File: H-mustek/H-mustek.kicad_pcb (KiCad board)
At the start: 2 copper layers, 22 parts, among them J1 Conn_01x02_Pin, J2 Conn_01x02_Pin, Q1 IRF3205, Q2 IRF3205, Q3 IRF3205, Q4 IRF3205, U1 IR2153, U2 IR2153

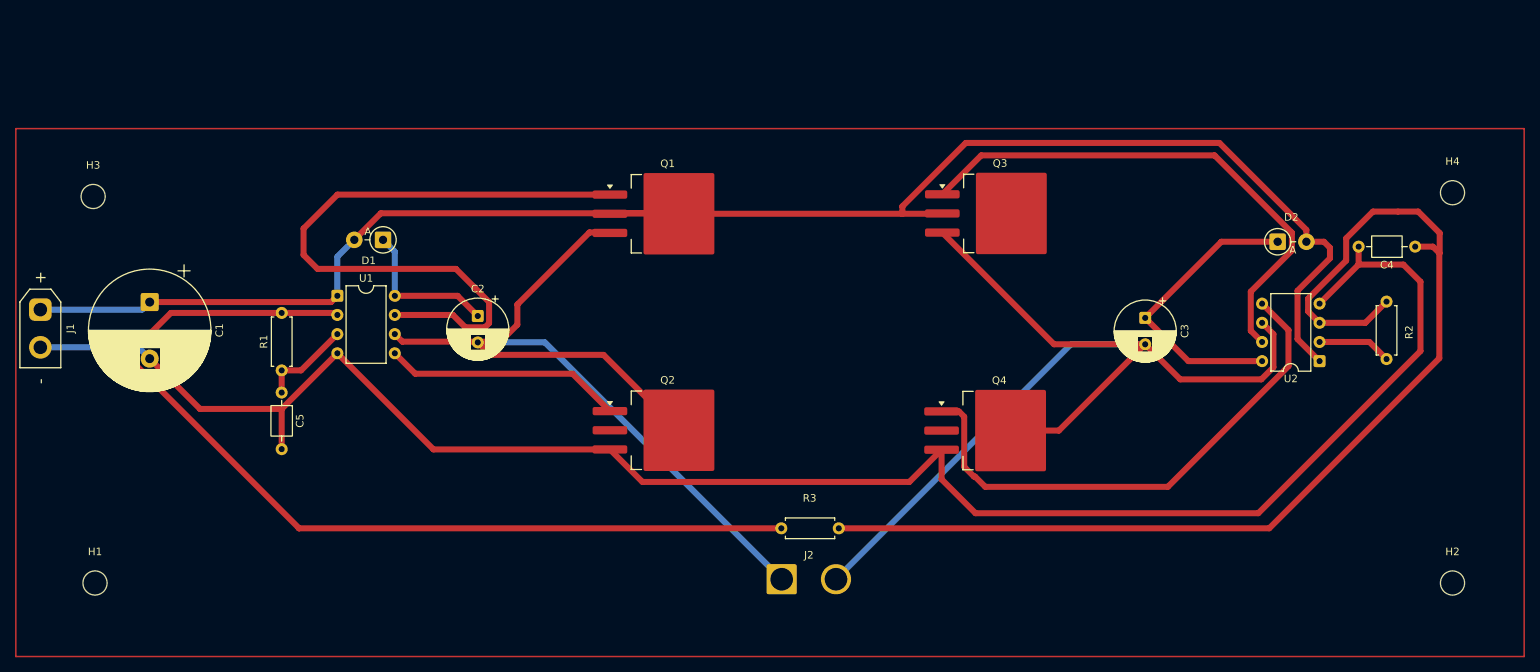
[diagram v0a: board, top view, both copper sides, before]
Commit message: 210426
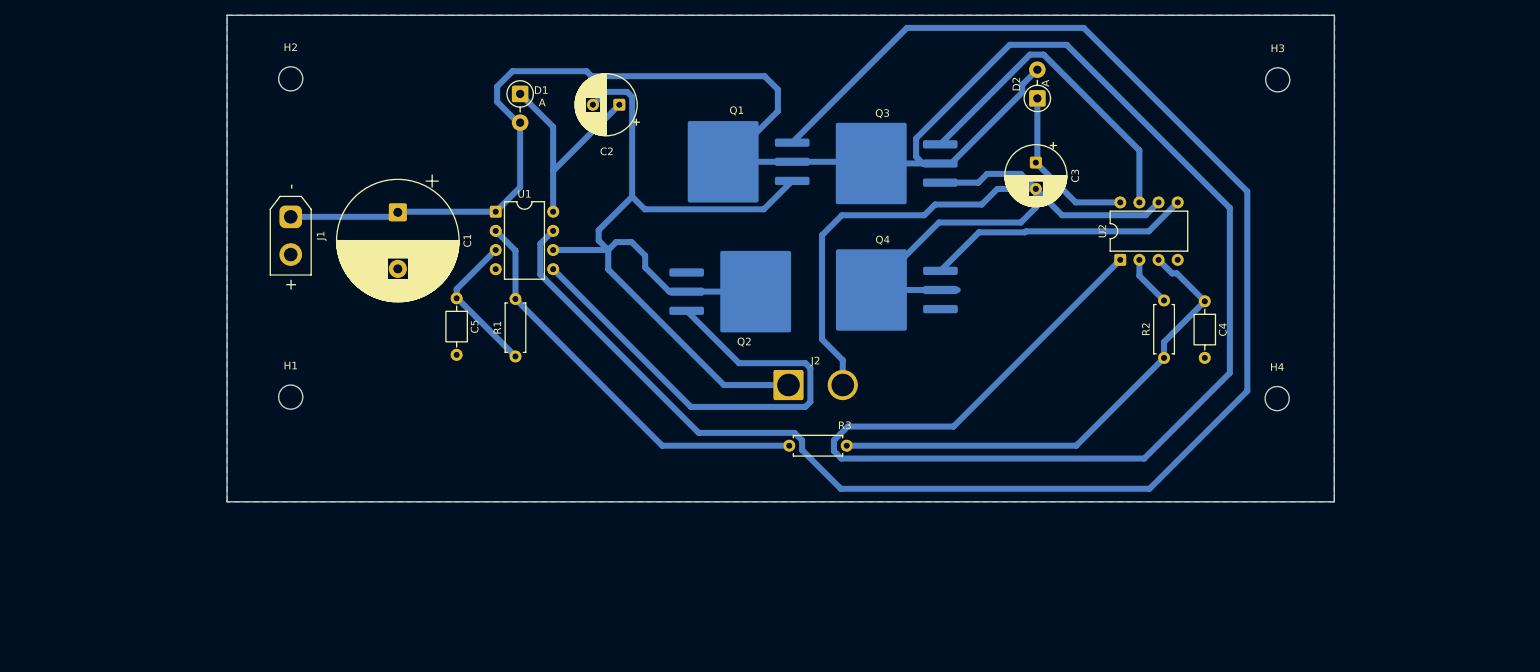
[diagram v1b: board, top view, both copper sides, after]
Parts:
- Q1, Q2, Q3, Q4: moved to B.Cu
- moved H2 167.9 mm to (104.2, 57.4)
- moved H3 157.8 mm to (235.1, 57.5)
- moved D2 37.1 mm to (203.2, 60.0), turned to 90 degrees
- moved H4 35.9 mm to (235.0, 99.8)
- moved H1 35.8 mm to (104.2, 99.6)
- moved J1 35.4 mm to (104.2, 75.7)
- moved C1 35.0 mm to (118.4, 75.1)
- moved C2 33.7 mm to (147.8, 60.8), turned to 180 degrees
- moved R1 31.1 mm to (134.0, 94.2)
- moved R2 30.4 mm to (220.0, 94.4), turned to 90 degrees
- moved U2 29.6 mm to (214.2, 81.4), turned to 90 degrees
- moved C4 28.8 mm to (225.4, 86.9), turned to -90 degrees
- moved D1 26.6 mm to (134.6, 59.4), turned to -90 degrees
- moved C5 26.4 mm to (126.2, 86.5)
- moved J2 25.8 mm to (170.2, 98.0)
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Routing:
- net GND: track 246.3 -> 0.00 mm
- net Net-(Q1-G): track 89.4 -> 220.2 mm
- net /VCC: track 225.0 -> 336.8 mm
- net Net-(U2-CT): track 148.1 -> 65.0 mm
- net Net-(U1-RT): track 126.0 -> 54.5 mm
- net Net-(Q4-G): track 70.4 -> 35.2 mm
- net Net-(Q2-G): track 31.7 -> 66.0 mm
- net Net-(Q3-G): track 70.1 -> 43.5 mm
- net Net-(D2-K): track 39.6 -> 22.0 mm
- net /VOUT2: track 135.6 -> 124.5 mm
- net Net-(D1-K): track 20.2 -> 29.8 mm
- net Net-(U1-CT): track 12.3 -> 19.5 mm
- net /VOUT1: track 121.6 -> 117.5 mm
- net Net-(U2-RT): track 9.82 -> 6.74 mm
- added copper zone on B.Cu, net GND
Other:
- board outline added: 146.8 x 64.5 mm
